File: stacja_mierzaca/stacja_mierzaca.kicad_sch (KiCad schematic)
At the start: 4 parts, among them U1 ESP32-WROOM32-DEVKIT-V1-30P, U2 DS18B20, U3 Ai-Thinker-Ra-02

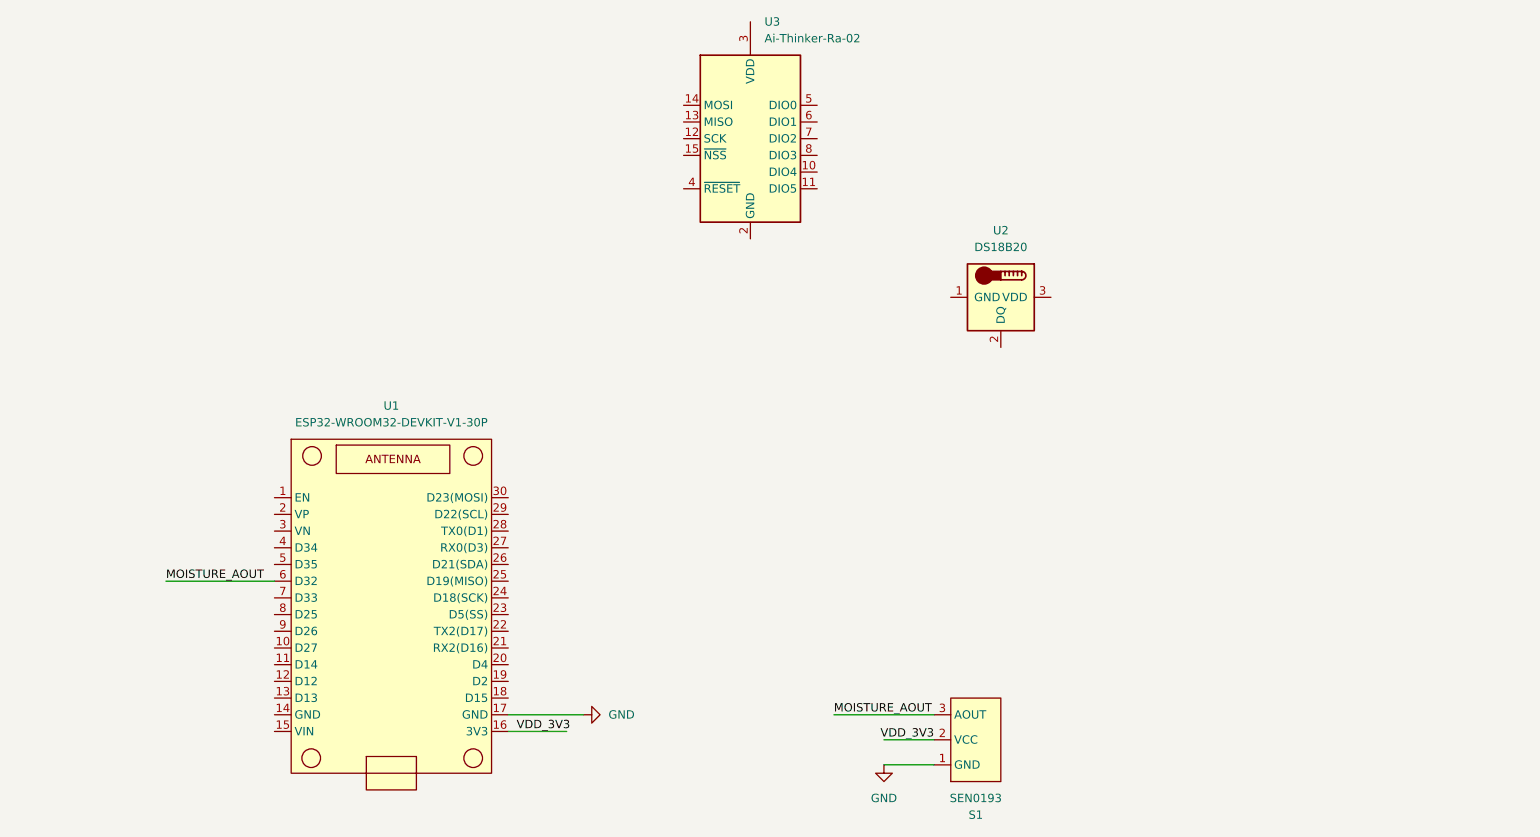
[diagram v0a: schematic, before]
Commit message: start of load sharing schematic
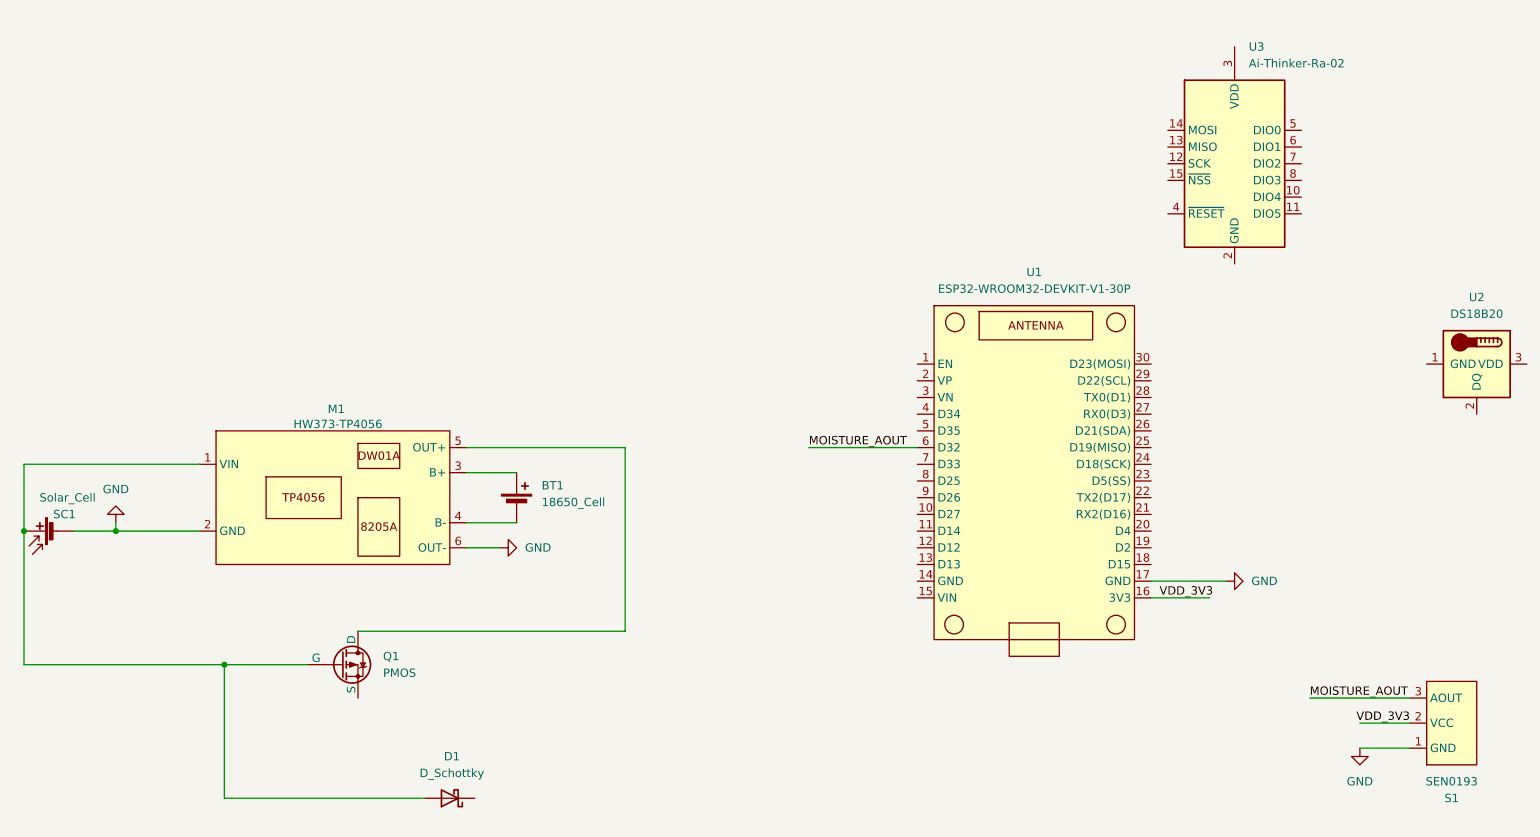
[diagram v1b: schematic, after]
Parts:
- added BT1: 18650_Cell, symbol Device:Battery_Cell
- added D1: D_Schottky, symbol Device:D_Schottky
- added M1: HW373-TP4056, symbol battery_management:HW373-TP4056
- added Q1: PMOS, symbol Simulation_SPICE:PMOS
- added SC1: Solar_Cell, symbol Device:Solar_Cell
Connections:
- net GND: now also M1.2 (GND), M1.6 (OUT-), SC1.2 (-)
- new net: D1.2 (A), M1.1 (VIN), Q1.2 (G), SC1.1 (+)
- new net: M1.5 (OUT+), Q1.1 (D)
- new net: BT1.1 (+), M1.3 (B+)
- new net: BT1.2 (-), M1.4 (B-)
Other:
- moved on the sheet: S1, U1, U2, U3
